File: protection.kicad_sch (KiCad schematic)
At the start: 17 parts, among them J4 Output, Q2 HY3610P, Q3 HY3610P

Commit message: finalised product
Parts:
- R31, R37, R38: footprint Resistor_THT:R_Axial_DIN0309_L9.0mm_D3.2mm_P15.24mm_Horizontal -> Resistor_SMD:R_1206_3216Metric
- R39: footprint Resistor_THT:R_Axial_DIN0309_L9.0mm_D3.2mm_P15.24mm_Horizontal -> Resistor_SMD:R_1210_3225Metric_Pad1.30x2.65mm_HandSolder
- R60: footprint Resistor_SMD:R_0603_1608Metric_Pad0.98x0.95mm_HandSolder -> Resistor_SMD:R_1206_3216Metric
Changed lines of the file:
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@@
 			)
 		)
-		(property "Footprint" "Resistor_THT:R_Axial_DIN0309_L9.0mm_D3.2mm_P15.24mm_Horizontal"
+		(property "Footprint" "Resistor_SMD:R_1206_3216Metric"
 			(at 116.332 118.11 90)
 			(effects
@@
 			)
 		)
-		(property "Footprint" "Resistor_THT:R_Axial_DIN0309_L9.0mm_D3.2mm_P15.24mm_Horizontal"
+		(property "Footprint" "Resistor_SMD:R_1206_3216Metric"
 			(at 85.852 113.03 90)
 			(effects
@@
 			)
 		)
-		(property "Footprint" "Resistor_SMD:R_0603_1608Metric_Pad0.98x0.95mm_HandSolder"
+		(property "Footprint" "Resistor_SMD:R_1206_3216Metric"
 			(at 85.852 123.19 90)
 			(effects
@@
 			)
 		)
-		(property "Footprint" "Resistor_THT:R_Axial_DIN0309_L9.0mm_D3.2mm_P15.24mm_Horizontal"
+		(property "Footprint" "Resistor_SMD:R_1206_3216Metric"
 			(at 116.332 127 90)
 			(effects
@@
 			)
 		)
-		(property "Footprint" "Resistor_THT:R_Axial_DIN0309_L9.0mm_D3.2mm_P15.24mm_Horizontal"
+		(property "Footprint" "Resistor_SMD:R_1210_3225Metric_Pad1.30x2.65mm_HandSolder"
 			(at 139.192 97.79 90)
 			(effects

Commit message: near end
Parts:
- R39: footprint Resistor_SMD:R_1210_3225Metric_Pad1.30x2.65mm_HandSolder -> Resistor_THT:R_Axial_DIN0309_L9.0mm_D3.2mm_P15.24mm_Horizontal
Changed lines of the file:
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@@
 			)
 		)
-		(property "Footprint" "Resistor_SMD:R_1210_3225Metric_Pad1.30x2.65mm_HandSolder"
+		(property "Footprint" "Resistor_THT:R_Axial_DIN0309_L9.0mm_D3.2mm_P15.24mm_Horizontal"
 			(at 139.192 97.79 90)
 			(effects

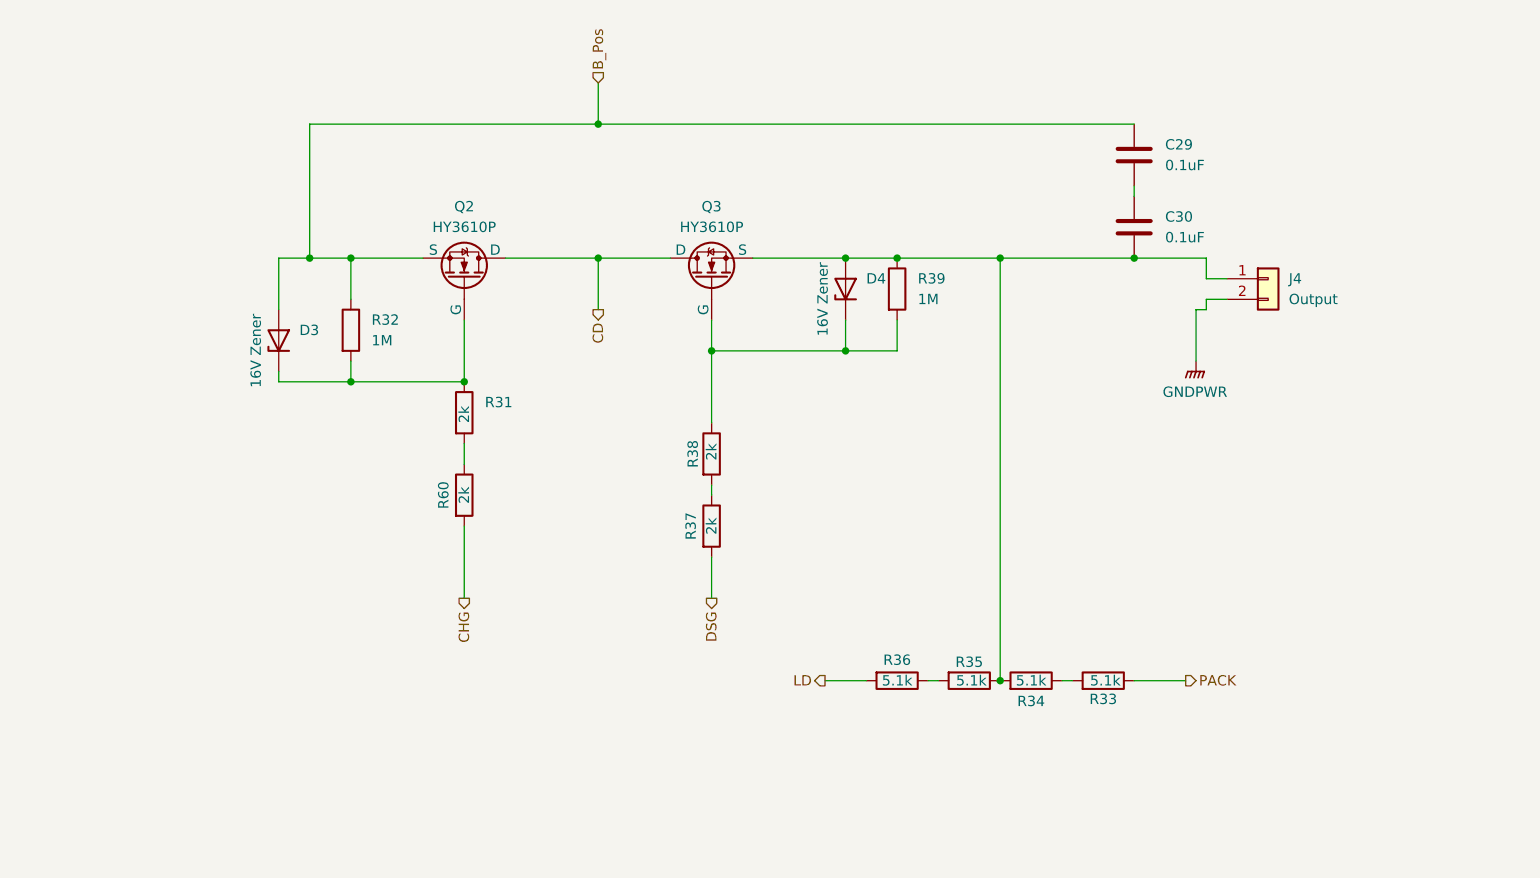
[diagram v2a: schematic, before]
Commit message: bit artık
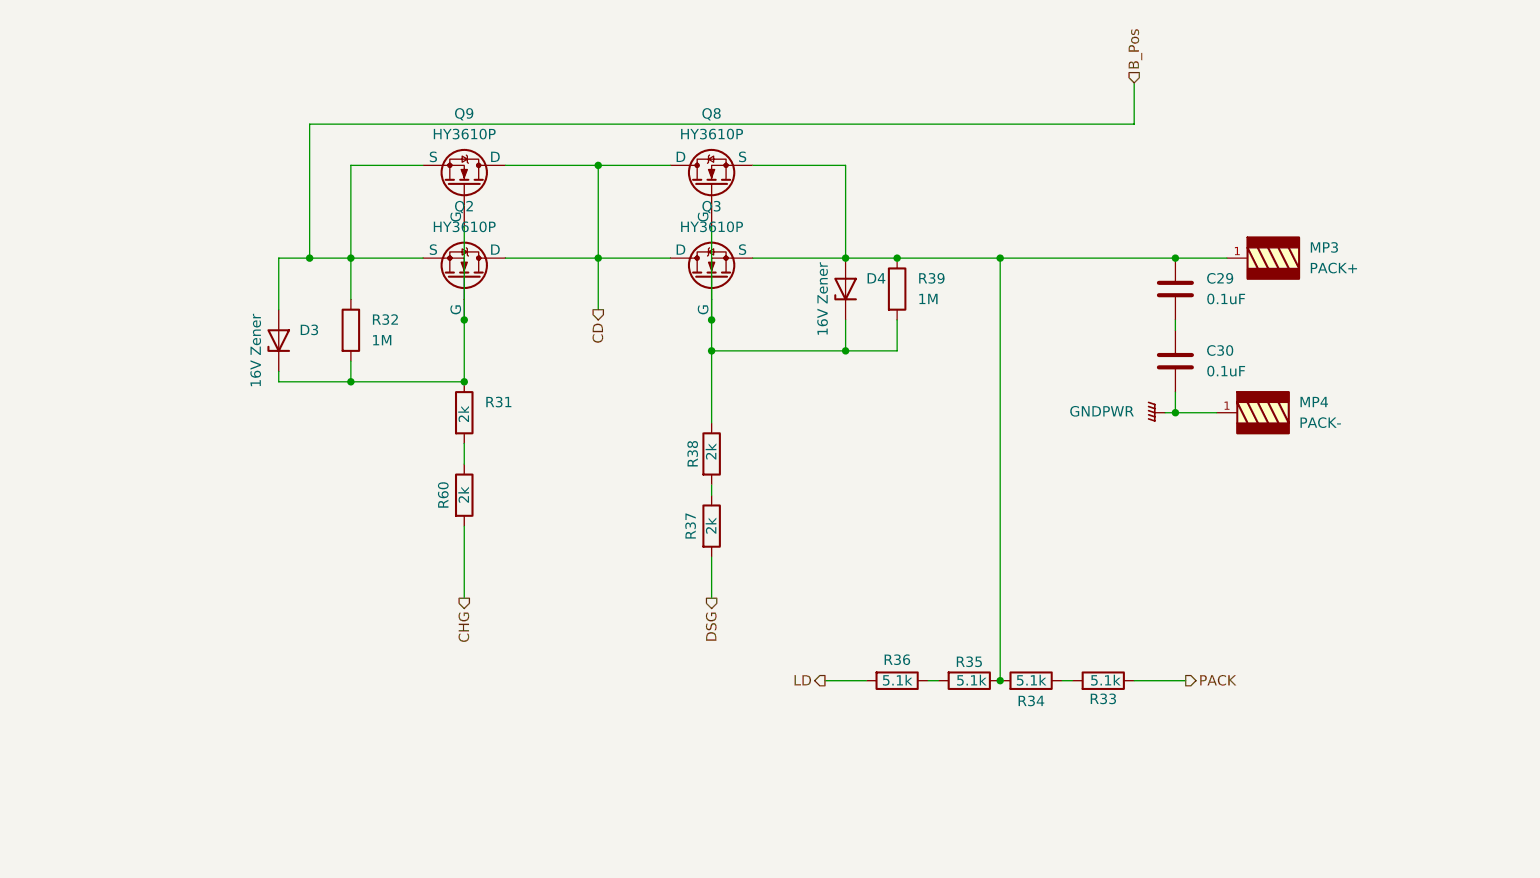
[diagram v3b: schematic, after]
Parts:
- removed J4: Output, Connector_AMASS:AMASS_XT60-F_1x02_P7.20mm_Vertical, symbol Connector_Generic:Conn_01x02
- added MP3: PACK+, WP-BUTR_7460307:WP-BUTR_7460307, symbol WP-BUTR:WP-BUTR
- added MP4: PACK-, WP-BUTR_7460307:WP-BUTR_7460307, symbol WP-BUTR:WP-BUTR
- added Q8, Q9: HY3610P, Package_TO_SOT_THT:TO-220-3_Vertical, symbol Simulation_SPICE:NMOS
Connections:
- net B_Pos: now also Q9.3 (S); no longer C29.1
- net CD: now also Q8.1 (D), Q9.1 (D)
- net GNDPWR: now also C30.2, MP4.1, MP4.2, MP4.3, MP4.4, MP4.5, MP4.6, MP4.7, MP4.8
- net at D4.2 (A), Q3.3 (S), R34.2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: now also C29.1, MP3.1, MP3.2, MP3.3, MP3.4, MP3.5, MP3.6, MP3.7, MP3.8, Q8.3 (S); no longer C30.2
- net at D4.1 (K), Q3.2 (G), R38.1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: now also Q8.2 (G)
- net at D3.1 (K), Q2.2 (G), R31.1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: now also Q9.2 (G)
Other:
- moved on the sheet: C29, C30

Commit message: BMS DONE IHOPE
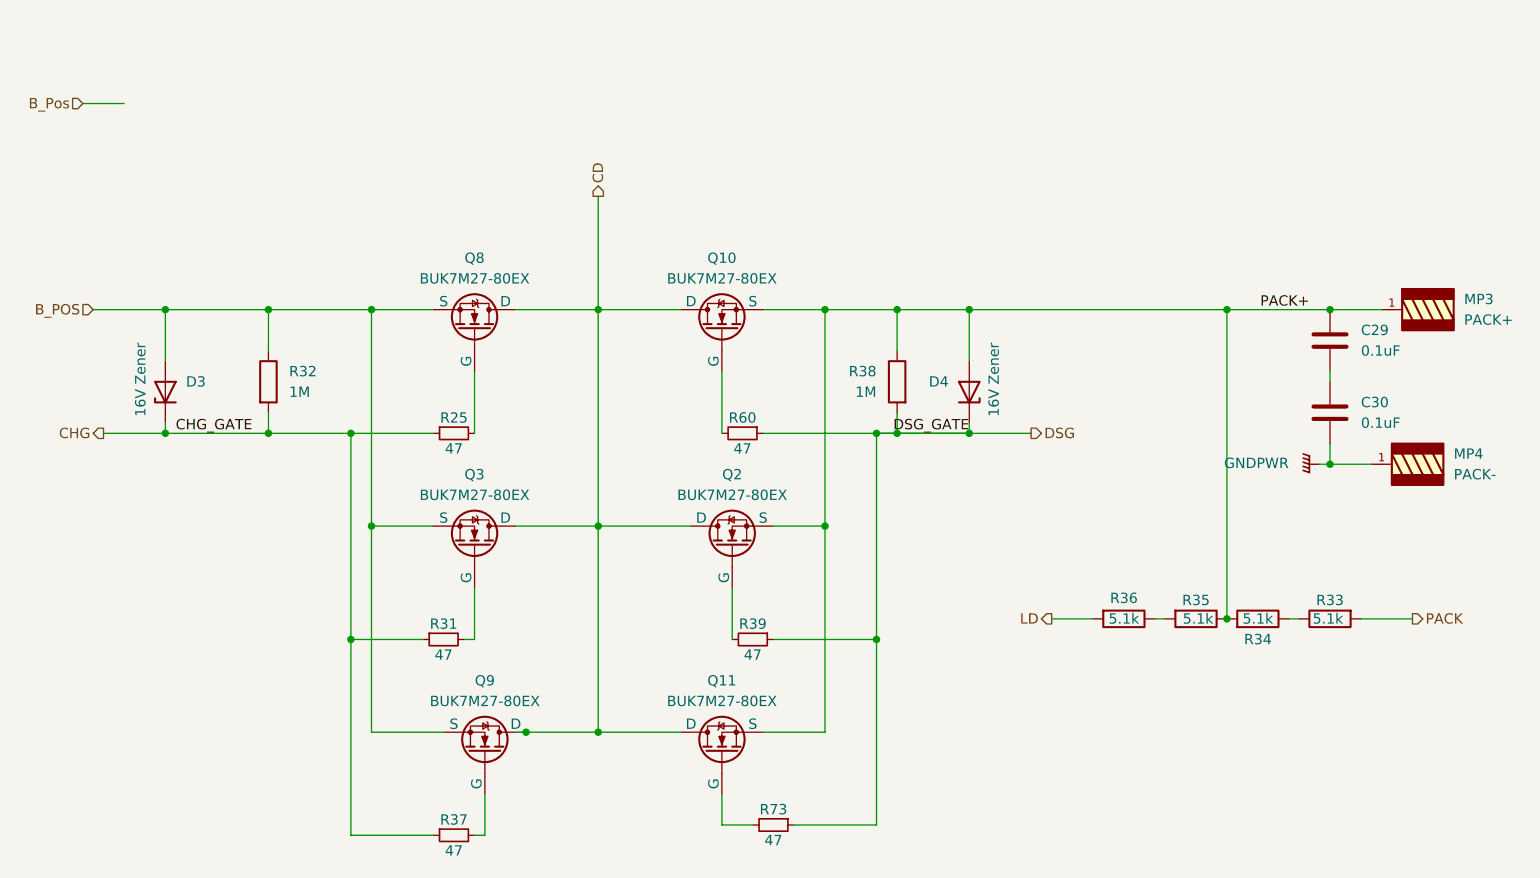
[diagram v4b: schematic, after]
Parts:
- removed R31, R37, R60: 2k, Resistor_SMD:R_1206_3216Metric, symbol Device:R
- removed R39: 1M, Resistor_THT:R_Axial_DIN0309_L9.0mm_D3.2mm_P15.24mm_Horizontal, symbol Device:R
- added Q10, Q11: BUK7M27-80EX, Package_TO_SOT_SMD:LFPAK33, symbol Simulation_SPICE:NMOS
- added R25, R31, R37, R39, R60, R73: 47, Resistor_SMD:R_0603_1608Metric_Pad0.98x0.95mm_HandSolder, symbol LibreSolar:R
- D3, D4: footprint Diode_THT:D_DO-201_P15.24mm_Horizontal -> Diode_SMD:D_SMF
- Q2, Q3, Q8, Q9: value HY3610P -> BUK7M27-80EX; footprint Package_TO_SOT_THT:TO-220-3_Vertical -> Package_TO_SOT_SMD:LFPAK33
- R32: footprint Resistor_THT:R_Axial_DIN0309_L9.0mm_D3.2mm_P15.24mm_Horizontal -> Resistor_SMD:R_2512_6332Metric_Pad1.40x3.35mm_HandSolder
- R33, R34, R35, R36: footprint Resistor_SMD:R_0508_1220Metric_Pad1.12x2.15mm_HandSolder -> Resistor_SMD:R_0603_1608Metric_Pad0.98x0.95mm_HandSolder
- R38: value 2k -> 1M; footprint Resistor_SMD:R_1206_3216Metric -> Resistor_SMD:R_2512_6332Metric_Pad1.40x3.35mm_HandSolder
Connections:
- net B_Pos: no longer D3.2 (A), Q2.3 (S), Q9.3 (S), R32.1
- net CD: now also Q2.5 (D), Q3.5 (D), Q8.5 (D), Q9.5 (D), Q10.5 (D), Q11.5 (D); no longer Q2.1 (D), Q3.1 (D), Q8.1 (D), Q9.1 (D)
- net CHG: now also D3.1 (K), R32.2, R25.1, R31.1, R37.1
- net DSG: now also D4.1 (K), R38.2, R39.1, R60.1, R73.1
- net PACK: now also R33.2; no longer R33.1
- net at R34.1: now also R33.1; no longer R33.2
- net PACK+: now reaches C29.1, D4.2 (A), MP3.1, MP3.2, MP3.3, MP3.4, MP3.5, MP3.6, MP3.7, MP3.8, R34.2, R35.1
- net PACK+: now also Q2.1 (S), Q2.2 (S), Q2.3 (S), R38.1, Q10.1 (S), Q10.2 (S), Q10.3 (S), Q11.1 (S), Q11.2 (S), Q11.3 (S); no longer Q3.3 (S), Q8.3 (S)
- net B_POS: now reaches Q3.2 (S), Q8.2 (S)
- net B_POS: now also D3.2 (A), Q3.1 (S), Q3.3 (S), Q8.1 (S), Q8.3 (S), Q9.1 (S), Q9.2 (S), Q9.3 (S), R32.1; no longer D4.1 (K), R38.1
- new net: Q11.4 (G), R73.2
- new net: Q8.4 (G), R25.2
- new net: Q2.4 (G), R39.2
- new net: Q3.4 (G), R31.2
- new net: Q10.4 (G), R60.2
- new net: Q9.4 (G), R37.2
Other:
- moved on the sheet: C29, C30, D3, MP3, MP4, R32, R33, R34, R35, R36
